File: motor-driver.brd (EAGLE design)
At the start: 33.4 x 42.7 mm, 37 parts, among them IC1 IR4427, IC2 IR4427, IC3 IR4427, IC5 ACS712-LC, Q1 IRF7389, Q2 IRF7389, Q3 IRF7389

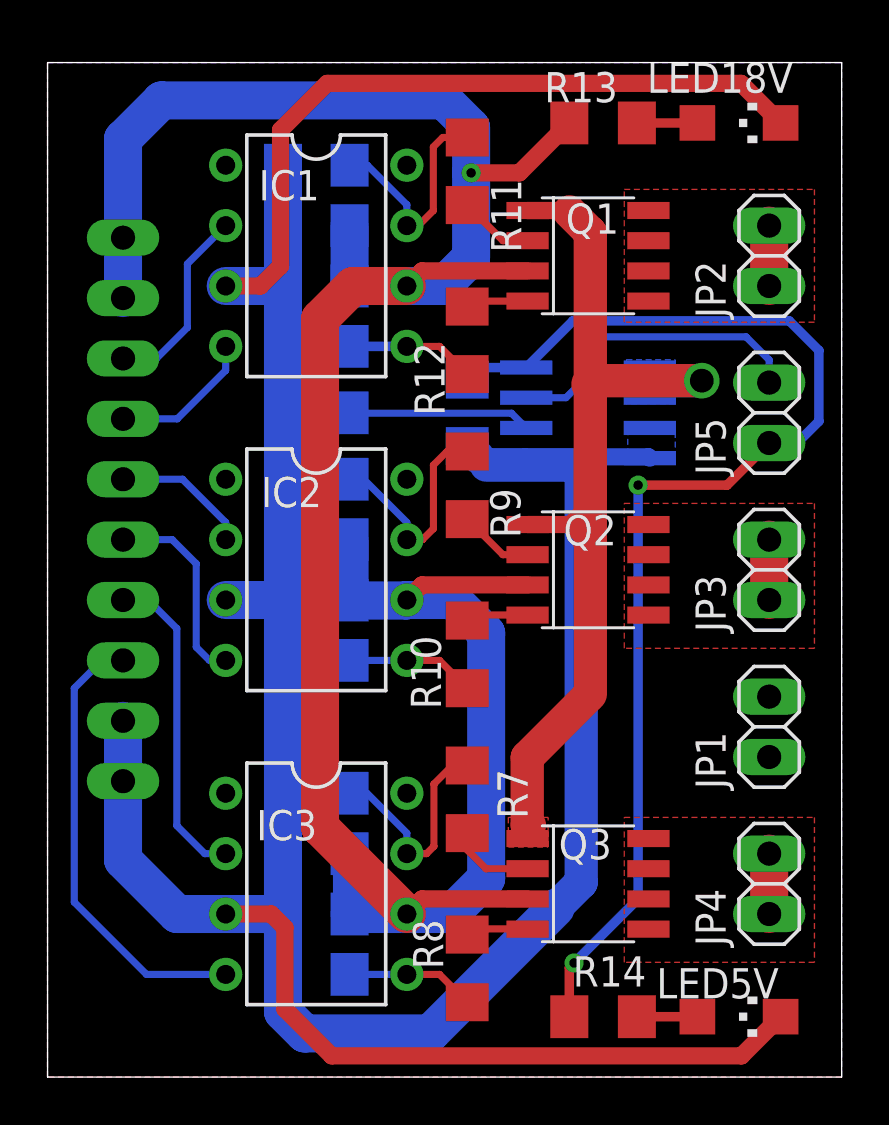
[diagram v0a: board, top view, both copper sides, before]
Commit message: applied some finishing touch
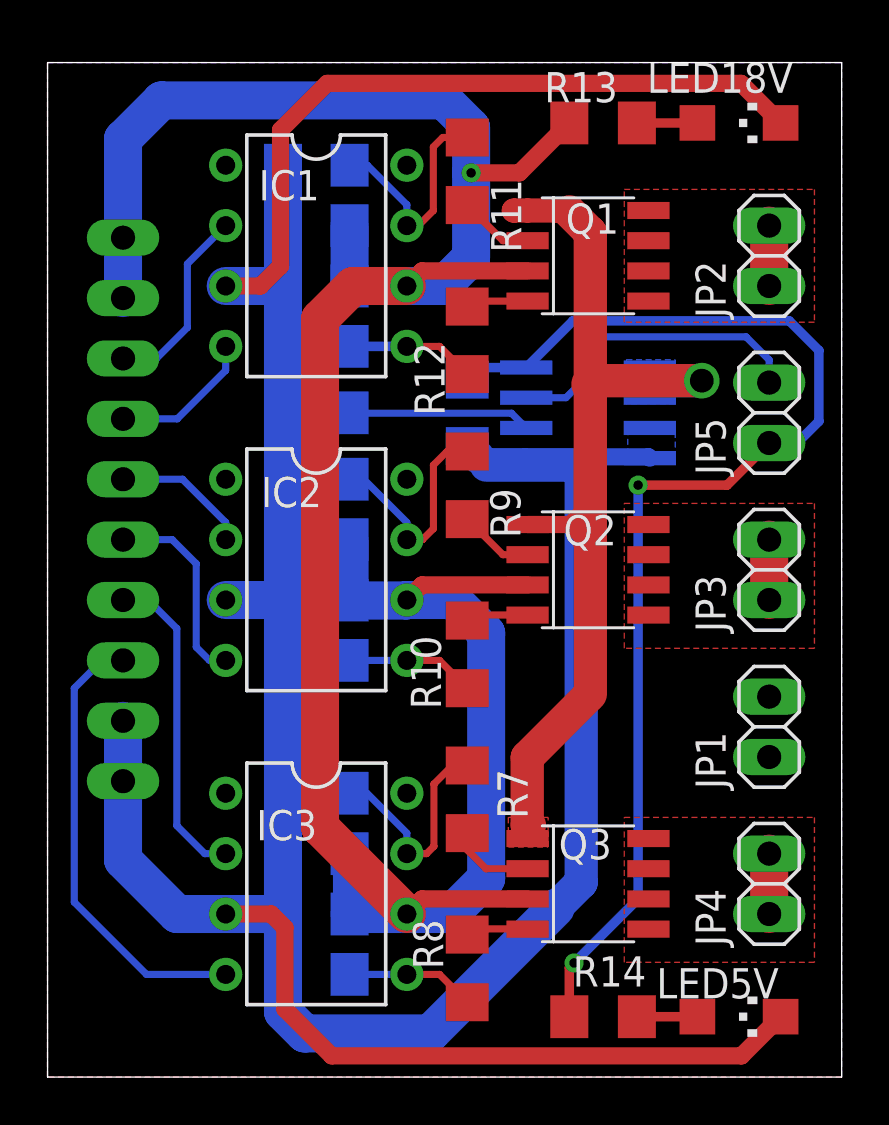
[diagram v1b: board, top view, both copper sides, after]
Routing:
- net SINK: track 41.0 -> 41.5 mm
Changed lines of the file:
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@@
 <setting verticaltext="up"/>
 </settings>
-<grid distance="50" unitdist="mil" unit="mil" style="lines" multiple="1" display="no" altdistance="5" altunitdist="mil" altunit="mil"/>
+<grid distance="0.000123031496" unitdist="mil" unit="mil" style="lines" multiple="1" display="no" altdistance="5" altunitdist="mil" altunit="mil"/>
 <layers>
 <layer number="1" name="Top" color="4" fill="1" visible="yes" active="yes"/>
@@
 <via x="31.91309375" y="48.9556" extent="1-16" drill="0.4"/>
 <wire x1="17.272" y1="43.688" x2="17.272" y2="46.228" width="1.6" layer="16"/>
-<wire x1="29.21" y1="17.78" x2="25.558453125" y2="21.431546875" width="1.6" layer="1"/>
+<wire x1="25.558453125" y1="21.431546875" x2="29.21" y2="17.78" width="1.6" layer="1"/>
 <wire x1="25.558453125" y1="21.431546875" x2="25.558453125" y2="42.810909375" width="1.6" layer="1"/>
 <wire x1="25.558453125" y1="42.810909375" x2="26.94354375" y2="44.196" width="1.6" layer="1"/>
@@
 <wire x1="36.5428375" y1="36.661834375" x2="36.5428375" y2="19.111178125" width="1.4" layer="16"/>
 <wire x1="31.75" y1="37.462" x2="32.201071875" y2="37.010928125" width="1.4" layer="16"/>
-<polygon width="0.3" layer="16" isolate="0.381" orphans="yes" rank="2">
+<polygon width="0.3" layer="16" isolate="0.381" rank="2">
 <vertex x="14.097" y="53.594"/>
 <vertex x="47.498" y="53.594"/>
@@
 <vertex x="14.097" y="10.922"/>
 </polygon>
-<polygon width="0.3" layer="1" isolate="0.381" orphans="yes" rank="2">
+<polygon width="0.3" layer="1" isolate="0.381" rank="2">
 <vertex x="14.097" y="53.594"/>
 <vertex x="47.498" y="53.594"/>
@@
 <wire x1="36.928090625" y1="27.02470625" x2="36.827384375" y2="26.924" width="0.725" layer="1"/>
 <wire x1="36.92645" y1="33.337096875" x2="36.928090625" y2="33.33545625" width="1.4" layer="1"/>
-<wire x1="36.92645" y1="46.43970625" x2="36.92645" y2="40.21409375" width="1.4" layer="1"/>
+<wire x1="36.92645" y1="40.21409375" x2="36.92645" y2="46.43970625" width="1.4" layer="1"/>
 <wire x1="36.92645" y1="40.06593125" x2="36.92645" y2="35.390334375" width="1.4" layer="1"/>
 <wire x1="36.92645" y1="35.390334375" x2="36.92645" y2="33.337096875" width="1.4" layer="1"/>
@@
 <wire x1="36.92645" y1="34.988903125" x2="36.92645" y2="35.390334375" width="0.75" layer="1"/>
 <wire x1="36.100546875" y1="34.163" x2="36.928090625" y2="33.33545625" width="0.75" layer="1"/>
-<wire x1="34.2868" y1="47.371" x2="35.99515625" y2="47.371" width="0.725" layer="1"/>
-<wire x1="36.04861875" y1="47.3175375" x2="36.92645" y2="46.43970625" width="1.4" layer="1"/>
+<wire x1="36.92645" y1="46.43970625" x2="36.04861875" y2="47.3175375" width="1.4" layer="1"/>
 <wire x1="35.99515625" y1="47.371" x2="36.04861875" y2="47.3175375" width="0.725" layer="1"/>
 <contactref element="IC5" pad="1"/>
@@
 <wire x1="41.616190625" y1="40.21409375" x2="39.343009375" y2="40.21409375" width="1.4" layer="16"/>
 <wire x1="39.343009375" y1="40.21409375" x2="39.343009375" y2="40.234453125" width="1.4" layer="16"/>
+<wire x1="34.2868" y1="47.371" x2="35.427815625" y2="47.371" width="1.016" layer="1"/>
+<wire x1="35.427815625" y1="47.371" x2="35.99515625" y2="47.371" width="1.016" layer="1"/>
+<wire x1="34.2868" y1="47.371" x2="33.70699375" y2="47.371" width="1.016" layer="1"/>
+<wire x1="33.70699375" y1="47.371" x2="33.70699375" y2="47.363928125" width="1.016" layer="1"/>
 </signal>
 <signal name="ACS_OUT">

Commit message: update motor-driver.brd
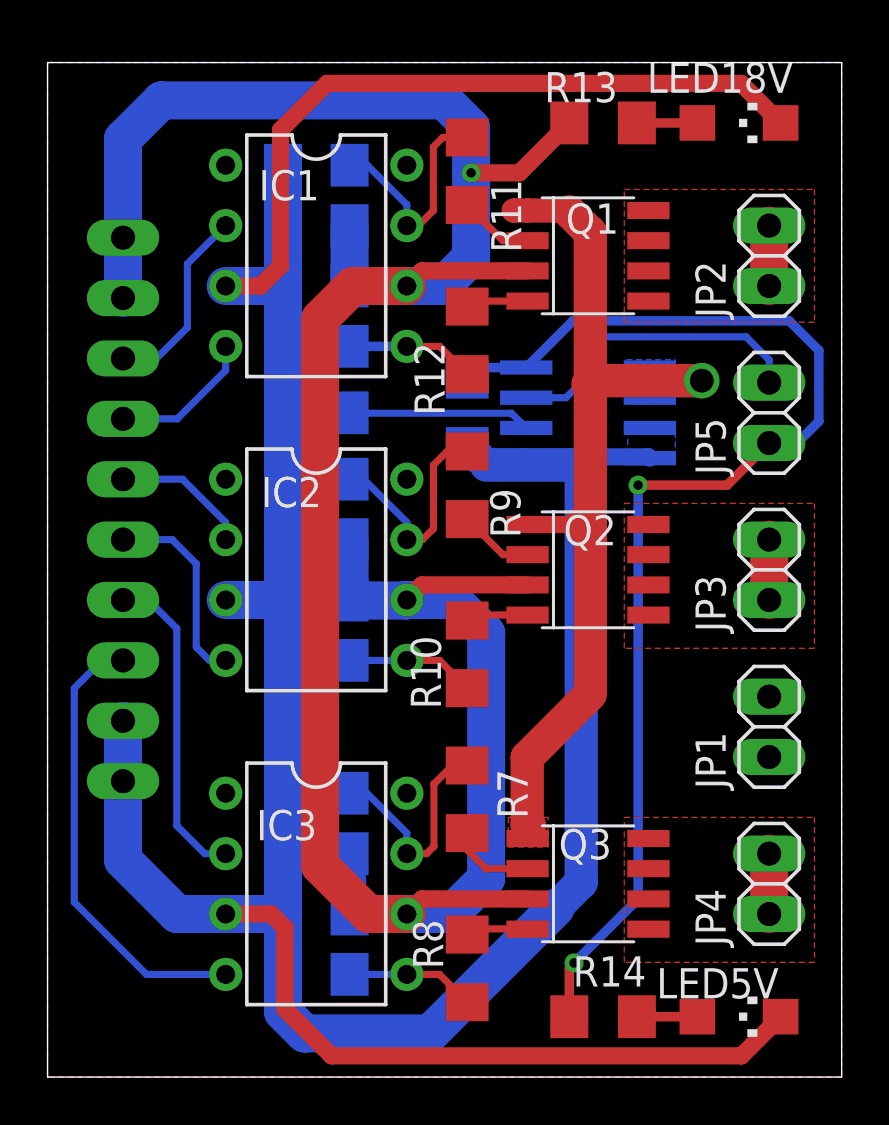
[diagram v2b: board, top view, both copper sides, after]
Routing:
- net VCC_18: track 116.0 -> 116.9 mm
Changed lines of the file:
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@@
 <via x="31.91309375" y="48.9556" extent="1-16" drill="0.4"/>
 <wire x1="17.272" y1="43.688" x2="17.272" y2="46.228" width="1.6" layer="16"/>
-<wire x1="25.558453125" y1="21.431546875" x2="29.21" y2="17.78" width="1.6" layer="1"/>
-<wire x1="25.558453125" y1="21.431546875" x2="25.558453125" y2="42.810909375" width="1.6" layer="1"/>
+<wire x1="27.59495625" y1="17.78" x2="29.21" y2="17.78" width="1.6" layer="1"/>
+<wire x1="27.59495625" y1="17.78" x2="25.558453125" y2="19.816503125" width="1.6" layer="1"/>
+<wire x1="25.558453125" y1="19.816503125" x2="25.558453125" y2="42.810909375" width="1.6" layer="1"/>
 <wire x1="25.558453125" y1="42.810909375" x2="26.94354375" y2="44.196" width="1.6" layer="1"/>
 <wire x1="26.94354375" y1="44.196" x2="29.21" y2="44.196" width="1.6" layer="1"/>
